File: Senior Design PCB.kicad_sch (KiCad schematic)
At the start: 60 parts, among them J1 Conn_01x02, J2 Conn_01x02, J3 Raspberry_Pi_Zero_2W, J7-1 Conn_01x04, J7-2 Conn_01x04, U1 LM2678SX-5.0/NOPB, U2 MCP3008, U3 MAX38890

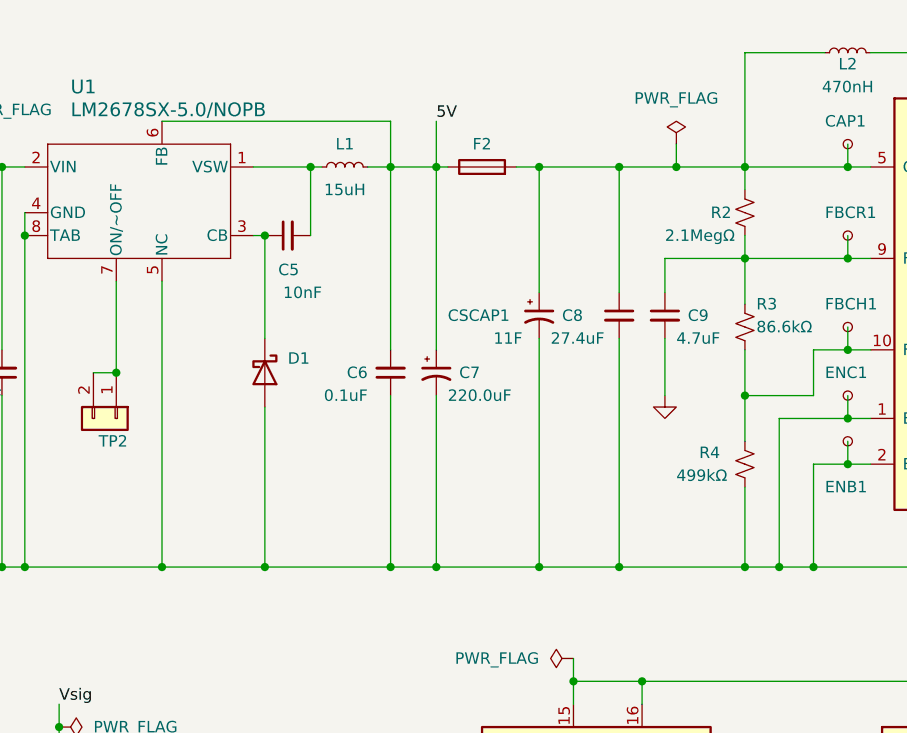
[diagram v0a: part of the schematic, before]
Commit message: Fixed a few footprints. Started the design process. I'll start making branches after today.
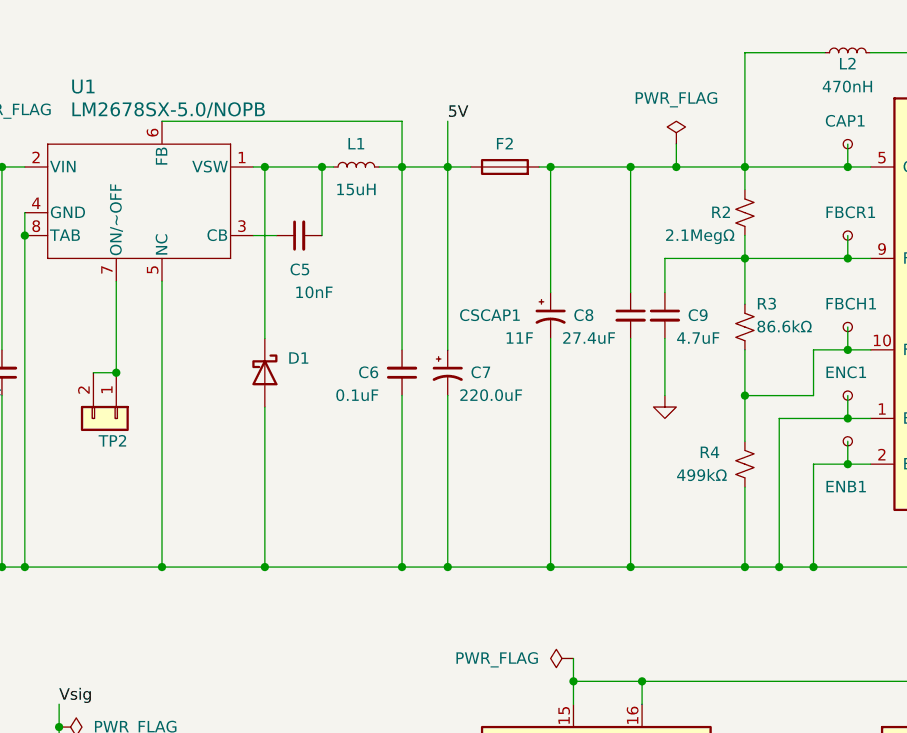
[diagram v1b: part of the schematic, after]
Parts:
- BKB1, CAP1, ENB1, ENC1, FBCH1, FBCR1, FBS1, ISET1, LX1, RDY1, SYS1: footprint Connector_Wire:SolderWire-1sqmm_1x02_P5.4mm_D1.4mm_OD2.7mm -> TestPoint:TestPoint_Pad_D2.0mm
- H1, H2, H3, H4: footprint MountingHole:MountingHole_5mm -> MountingHole:MountingHole_5.3mm_M5_Pad
- H5, H6, H7, H8: footprint MountingHole:MountingHole_3.5mm -> MountingHole:MountingHole_3.5mm_Pad
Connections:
- net at C5.2, L1.1, U1.1 (VSW): now also D1.1 (K)
- net at C5.1, U1.3 (CB): no longer D1.1 (K)
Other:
- moved on the sheet: C5, C6, C7, C8, CSCAP1, F2, L1
